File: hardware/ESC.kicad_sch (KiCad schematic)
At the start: 1 part, among them U1 DRV8323HRTAR

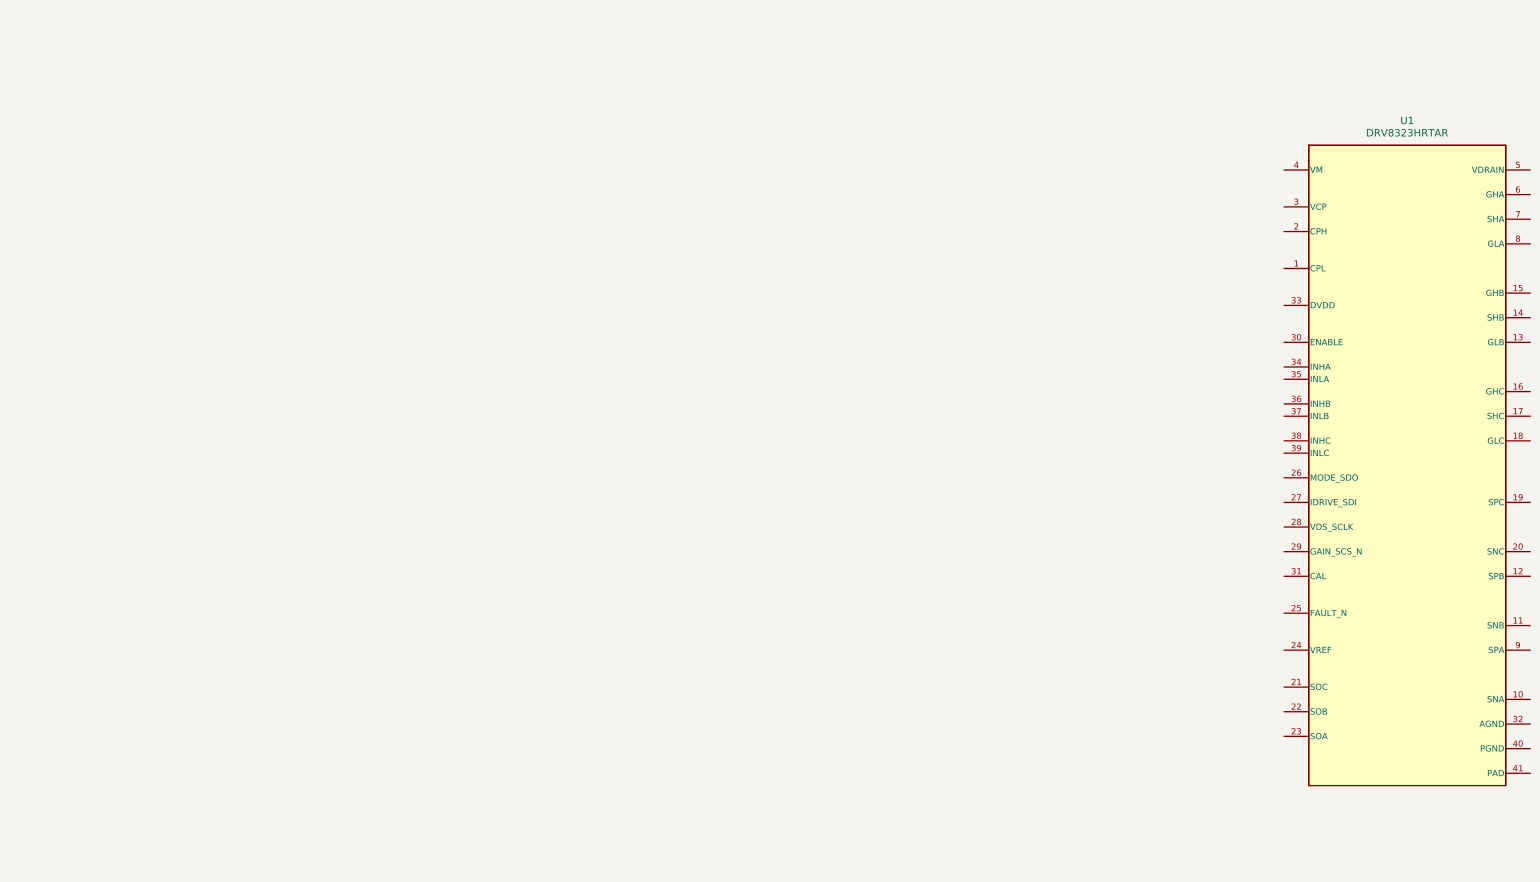
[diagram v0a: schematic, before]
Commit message: started schematic
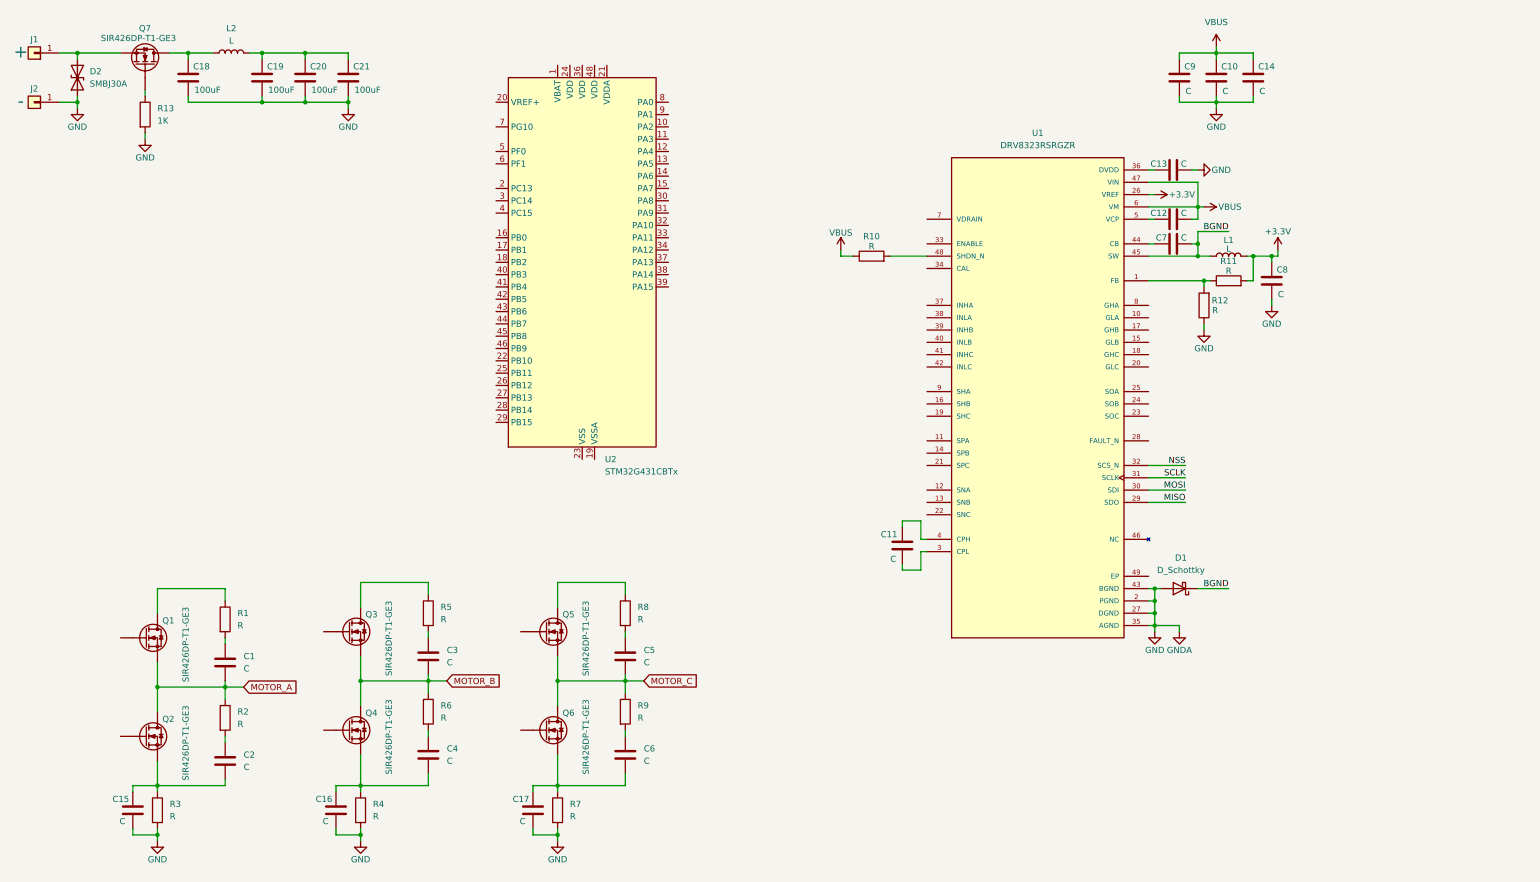
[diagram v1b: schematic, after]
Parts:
- removed U1: DRV8323HRTAR, RTA0040B, symbol ESC-Imports:DRV8323HRTAR
- added C1, C10, C11, C12, C13, C14, C15, C16, C17, C2, C3, C4, C5, C6, C7, C8, C9: C, symbol Device:C
- added C18, C19, C20, C21: 100uF, symbol Device:C
- added D1: D_Schottky, symbol Device:D_Schottky
- added D2: SMBJ30A, symbol Device:D_TVS
- added J1: +, symbol Connector_Generic:Conn_01x01
- added J2: -, symbol Connector_Generic:Conn_01x01
- added L1, L2: L, symbol Device:L
- added Q1, Q2, Q3, Q4, Q5, Q6, Q7: SIR426DP-T1-GE3, symbol Device:Q_NMOS
- added R1, R10, R11, R12, R2, R3, R4, R5, R6, R7, R8, R9: R, symbol Device:R
- added R13: 1K, symbol Device:R
- added U1: DRV8323RSRGZR, DRV8323RSRGZR:QFN50P700X700X100-49N, symbol ESC-Imports:DRV8323RSRGZR
- added U2: STM32G431CBTx, Package_QFP:LQFP-48_7x7mm_P0.5mm, symbol MCU_ST_STM32G4:STM32G431CBTx
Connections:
- new net: C19.1, C20.1, C21.1, L2.2
- new net: Q5.D, R8.1
- new net: C13.1, U1.36 (DVDD)
- new net: R11.1, R12.2, U1.1 (FB)
- new net: C11.1, U1.4 (CPH)
- new net: C11.2, U1.3 (CPL)
- new net: C18.1, L2.1, Q7.D
- new net: Q3.D, R5.1
- new net: C16.1, C4.2, Q4.S, R4.1
- new net: C4.1, R6.2
- new net: C15.1, C2.2, Q2.S, R3.1
- new net: C3.1, R5.2
- new net: C2.1, R2.2
- new net: D2.2 (A2), J1.1 (Pin_1), Q7.S
- new net: C5.1, R8.2
- new net: C12.1, U1.5 (VCP)
- new net: U2.23 (VSS), U2.35 (VSS), U2.47 (VSS)
- new net: C7.1, U1.44 (CB)
- new net: Q7.G, R13.1
- new net: R10.2, U1.48 (SHDN_N)
- new net: C6.1, R9.2
- new net: C17.1, C6.2, Q6.S, R7.1
- new net: Q1.D, R1.1
- new net: C1.1, R1.2
- new net +3.3V: C8.1, L1.2, R11.2, U1.26 (VREF)
- new net BGND: C7.2, D1.1 (K), L1.1, U1.45 (SW)
- new net GND: C10.2, C13.2, C14.2, C15.2, C16.2, C17.2, C18.2, C19.2, C20.2, C21.2, C8.2, C9.2, D1.2 (A), D2.1 (A1), J2.1 (Pin_1), R12.1, R13.2, R3.2, R4.2, R7.2, U1.2 (PGND), U1.27 (DGND), U1.35 (AGND), U1.43 (BGND)
- new net MISO: U1.29 (SDO)
- new net MOSI: U1.30 (SDI)
- new net MOTOR_A: C1.2, Q1.S, Q2.D, R2.1
- new net MOTOR_B: C3.2, Q3.S, Q4.D, R6.1
- new net MOTOR_C: C5.2, Q5.S, Q6.D, R9.1
- new net NSS: U1.32 (SCS_N)
- new net SCLK: U1.31 (SCLK)
- new net VBUS: C10.1, C12.2, C14.1, C9.1, R10.1, U1.47 (VIN), U1.6 (VM)

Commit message: finished most of schematic
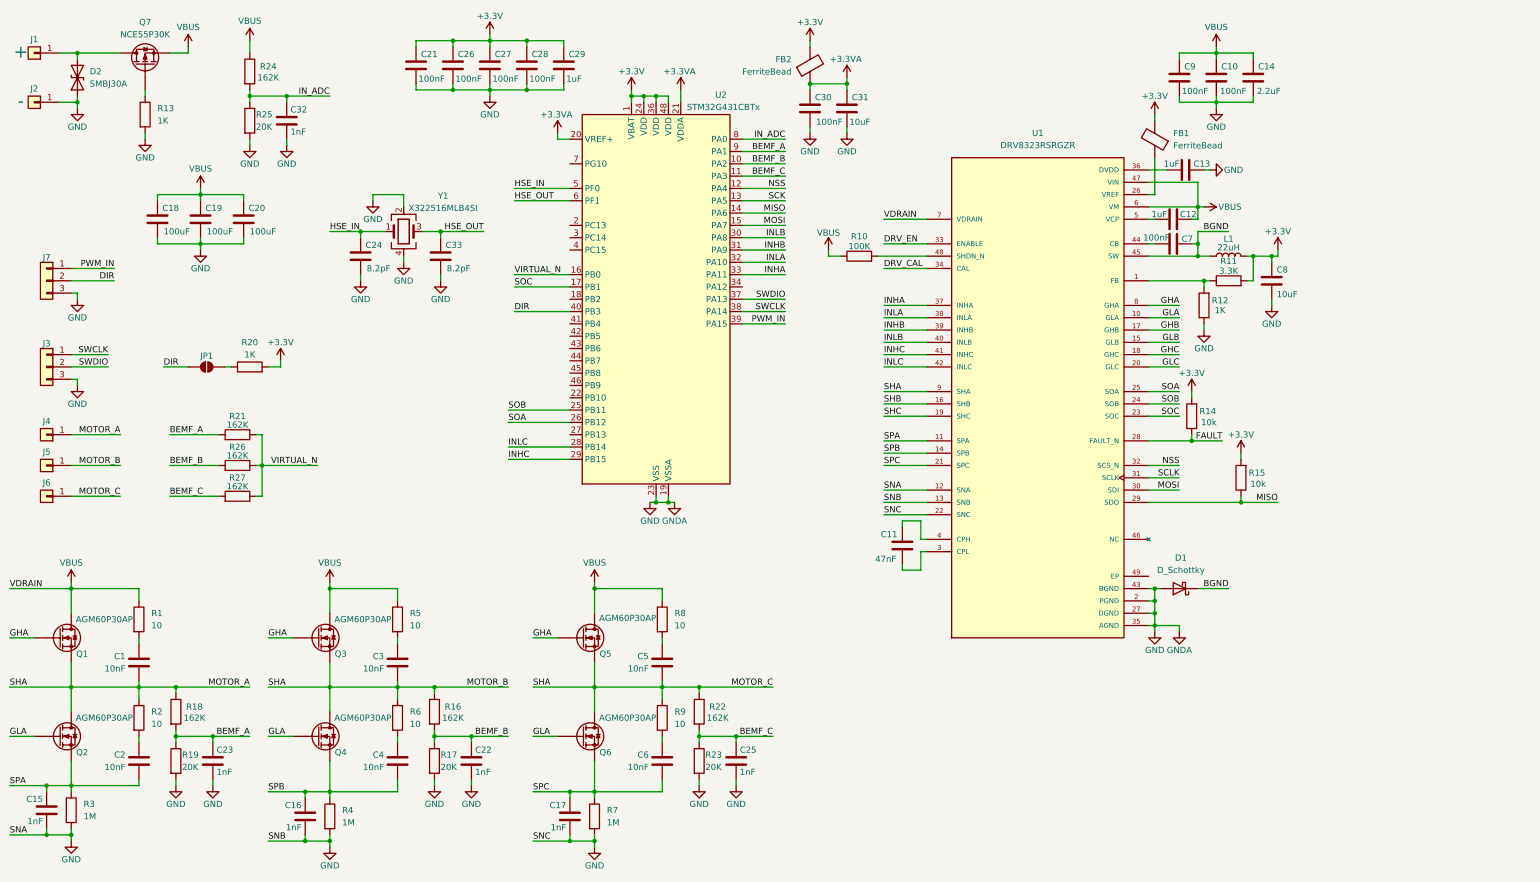
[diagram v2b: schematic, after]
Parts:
- removed L2: L, symbol Device:L
- removed Q7: SIR426DP-T1-GE3, symbol Device:Q_NMOS
- added C22, C23: 1nF, Capacitor_SMD:C_0603_1608Metric, symbol Device:C
- added C24, C33: 8.2pF, Capacitor_SMD:C_0402_1005Metric, symbol Device:C
- added C25, C32: 1nF, Capacitor_SMD:C_0402_1005Metric, symbol Device:C
- added C26, C27, C28, C30: 100nF, Capacitor_SMD:C_0402_1005Metric, symbol Device:C
- added C29: 1uF, Capacitor_SMD:C_0402_1005Metric, symbol Device:C
- added C31: 10uF, Capacitor_SMD:C_0402_1005Metric, symbol Device:C
- added FB1, FB2: FerriteBead, Inductor_SMD:L_0603_1608Metric, symbol Device:FerriteBead
- added J3, J7: Conn_01x03, Connector_PinHeader_2.54mm:PinHeader_1x03_P2.54mm_Vertical, symbol Connector_Generic:Conn_01x03
- added J4, J5, J6: +, Connector_Wire:SolderWire-4sqmm_1x01_D3mm_OD6mm, symbol Connector_Generic:Conn_01x01
- added JP1: SolderJumper_2_Open, Jumper:SolderJumper-2_P1.3mm_Open_RoundedPad1.0x1.5mm, symbol Jumper:SolderJumper_2_Open
- added Q7: NCE55P30K, Package_TO_SOT_SMD:TO-252-2, symbol Device:Q_PMOS
- added R14, R15: 10k, Resistor_SMD:R_0402_1005Metric, symbol Device:R
- added R16, R18, R21, R22, R24, R26, R27: 162K, Resistor_SMD:R_0402_1005Metric, symbol Device:R
- added R17, R19, R23, R25: 20K, Resistor_SMD:R_0402_1005Metric, symbol Device:R
- added R20: 1K, Resistor_SMD:R_0402_1005Metric, symbol Device:R
- added Y1: X322516MLB4SI, Crystal:Crystal_SMD_3225-4Pin_3.2x2.5mm, symbol Device:Crystal_GND24
- C1, C2, C3, C4, C5, C6: value C -> 10nF; footprint (none) -> Capacitor_SMD:C_0402_1005Metric
- C10, C7, C9: value C -> 100nF; footprint (none) -> Capacitor_SMD:C_0402_1005Metric
- C11: value C -> 47nF; footprint (none) -> Capacitor_SMD:C_0402_1005Metric
- C12, C13: value C -> 1uF; footprint (none) -> Capacitor_SMD:C_0402_1005Metric
- C14: value C -> 2.2uF; footprint (none) -> Capacitor_SMD:C_0402_1005Metric
- C15, C16, C17: value C -> 1nF; footprint (none) -> Capacitor_SMD:C_0402_1005Metric
- C18, C19, C20: footprint (none) -> Capacitor_SMD:C_Elec_6.3x7.7
- C21: value 100uF -> 100nF; footprint (none) -> Capacitor_SMD:C_0402_1005Metric
- C8: value C -> 10uF; footprint (none) -> Capacitor_SMD:C_0402_1005Metric
- D1: footprint (none) -> Diode_SMD:D_SOD-123
- D2: footprint (none) -> Diode_SMD:D_SMA
- J1, J2: footprint (none) -> Connector_Wire:SolderWire-4sqmm_1x01_D3mm_OD6mm
- L1: value L -> 22uH; footprint (none) -> Inductor_SMD:L_APV_ANR5012
- Q1, Q2, Q3, Q4, Q5, Q6: value SIR426DP-T1-GE3 -> AGM60P30AP; footprint (none) -> Package_DFN_QFN:PQFN-8-EP_6x5mm_P1.27mm_Generic
- R1, R2, R5, R6, R8, R9: value R -> 10; footprint (none) -> Resistor_SMD:R_0603_1608Metric
- R10: value R -> 100K; footprint (none) -> Resistor_SMD:R_0402_1005Metric
- R11: value R -> 3.3K; footprint (none) -> Resistor_SMD:R_0402_1005Metric
- R12: value R -> 1K; footprint (none) -> Resistor_SMD:R_0402_1005Metric
- R13: footprint (none) -> Resistor_SMD:R_0603_1608Metric
- R3, R4, R7: value R -> 1M; footprint (none) -> Resistor_SMD:R_1206_3216Metric
- U1: footprint DRV8323RSRGZR:QFN50P700X700X100-49N -> Package_DFN_QFN:QFN-48-1EP_7x7mm_P0.5mm_EP5.1x5.1mm_ThermalVias
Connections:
- net +3.3V: now also C21.1, U2.1 (VBAT), U2.24 (VDD), U2.36 (VDD), U2.48 (VDD), C26.1, C27.1, C28.1, C29.1, FB1.2, FB2.2, R14.2, R15.2, R20.2; no longer U1.26 (VREF)
- net GND: now also U1.12 (SNA), U1.13 (SNB), U1.22 (SNC), U2.19 (VSSA), U2.23 (VSS), U2.35 (VSS), U2.47 (VSS), C22.2, C23.2, C24.2, C25.2, C26.2, C27.2, C28.2, C29.2, C30.2, C31.2, C32.2, C33.2, J3.3 (Pin_3), J7.3 (Pin_3), R17.2, R19.2, R23.2, R25.2, Y1.2, Y1.4
- net MISO: now also U2.14 (PA6), R15.1
- net MOSI: now also U2.15 (PA7)
- net MOTOR_A: now also C3.2, C5.2, Q1.1 (S), Q2.3 (D), Q3.1 (S), Q4.3 (D), Q5.1 (S), Q6.3 (D), R6.1, R9.1, U1.9 (SHA), J4.1 (Pin_1), J5.1 (Pin_1), J6.1 (Pin_1), R16.1, R18.1, R22.1; no longer Q1.S, Q2.D
- net NSS: now also U2.12 (PA4)
- net VBUS: now also C18.1, C19.1, C20.1, Q1.3 (D), Q3.3 (D), Q5.3 (D), R1.1, R5.1, R8.1, U1.7 (VDRAIN), Q7.S, R24.1
- net SPB: now reaches C16.1, C4.2, R4.1
- net SPB: now also Q4.1 (S), U1.14 (SPB); no longer Q4.S
- net SPA: now reaches C15.1, C2.2, R3.1
- net SPA: now also Q2.1 (S), U1.11 (SPA); no longer Q2.S
- net at D2.2 (A2), J1.1 (Pin_1): now also Q7.D
- net BEMF_B: now reaches U2.10 (PA2)
- net BEMF_B: now also C22.1, R16.2, R17.1, R26.2
- net BEMF_C: now reaches U2.11 (PA3)
- net BEMF_C: now also C25.1, R22.2, R23.1, R27.2
- net SCK: now reaches U2.13 (PA5)
- net VIRTUAL_N: now reaches U2.16 (PB0)
- net VIRTUAL_N: now also R21.1, R26.1, R27.1
- net SOC: now reaches U2.17 (PB1)
- net SOC: now also U1.23 (SOC)
- net +3.3VA: now reaches U2.20 (VREF+)
- net +3.3VA: now also U2.21 (VDDA), C30.1, C31.1, FB2.1
- net SOB: now reaches U2.25 (PB11)
- net SOB: now also U1.24 (SOB)
- net SOA: now reaches U2.26 (PB12)
- net SOA: now also U1.25 (SOA)
- net INLC: now reaches U2.28 (PB14)
- net INLC: now also U1.42 (INLC)
- net INHC: now reaches U2.29 (PB15)
- net INHC: now also U1.41 (INHC)
- net INLB: now reaches U2.30 (PA8)
- net INLB: now also U1.40 (INLB)
- net INHB: now reaches U2.31 (PA9)
- net INHB: now also U1.39 (INHB)
- net INLA: now reaches U2.32 (PA10)
- net INLA: now also U1.38 (INLA)
- net INHA: now reaches U2.33 (PA11)
- net INHA: now also U1.37 (INHA)
- net SWDIO: now reaches U2.37 (PA13)
- net SWDIO: now also J3.2 (Pin_2)
- net SWCLK: now reaches U2.38 (PA14)
- net SWCLK: now also J3.1 (Pin_1)
- net PWM_IN: now reaches U2.39 (PA15)
- net PWM_IN: now also J7.1 (Pin_1)
- net DIR: now reaches U2.40 (PB3)
- net DIR: now also J7.2 (Pin_2), JP1.1 (A)
- net HSE_IN: now reaches U2.5 (PF0)
- net HSE_IN: now also C24.1, Y1.1
- net HSE_OUT: now reaches U2.6 (PF1)
- net HSE_OUT: now also C33.1, Y1.3
- net IN_ADC: now reaches U2.8 (PA0)
- net IN_ADC: now also C32.1, R24.2, R25.1
- net BEMF_A: now reaches U2.9 (PA1)
- net BEMF_A: now also C23.1, R18.2, R19.1, R21.2
- net at R13.1: now also Q7.G
- net GLA: now reaches U1.10 (GLA)
- net GLA: now also Q2.2 (G), Q4.2 (G), Q6.2 (G)
- net GLB: now reaches U1.15 (GLB)
- net SHB: now reaches U1.16 (SHB)
- net GHB: now reaches U1.17 (GHB)
- net GHC: now reaches U1.18 (GHC)
- net SHC: now reaches U1.19 (SHC)
- net GLC: now reaches U1.20 (GLC)
- net SPC: now reaches U1.21 (SPC)
- net SPC: now also C17.1, C6.2, Q6.1 (S), R7.1
- net FAULT: now reaches U1.28 (FAULT_N)
- net FAULT: now also R14.1
- net DRV_EN: now reaches U1.33 (ENABLE)
- net DRV_CAL: now reaches U1.34 (CAL)
- net GHA: now reaches U1.8 (GHA)
- net GHA: now also Q1.2 (G), Q3.2 (G), Q5.2 (G)
- removed net MOTOR_B: C3.2, Q3.S, Q4.D, R6.1
- removed net MOTOR_C: C5.2, Q5.S, Q6.D, R9.1
- new net: JP1.2 (B), R20.1
- new net: FB1.1, U1.26 (VREF)
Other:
- moved on the sheet: C1, C13, C15, C16, C17, C18, C19, C20, Q1, Q2, Q3, Q4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
